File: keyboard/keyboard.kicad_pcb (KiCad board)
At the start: 2 copper layers, 166.5 x 124 mm, 82 parts, among them J1 Conn_01x04, J2 Conn_01x04, SW1 SW_Push, SW10 SW_Push, SW11 SW_Push, SW12 SW_Push, SW13 SW_Push, SW14 SW_Push, SW15 SW_Push, SW16 SW_Push, SW17 SW_Push, SW18 SW_Push, SW19 SW_Push, SW2 SW_Push, SW20 SW_Push, SW21 SW_Push, SW3 SW_Push, SW4 SW_Push, SW5 SW_Push, SW6 SW_Push, SW7 SW_Push, SW8 SW_Push, SW9 SW_Push, U1 AP2127K-3.3, U2 USBLC6-2SC6, U3 STM32F072CBTx

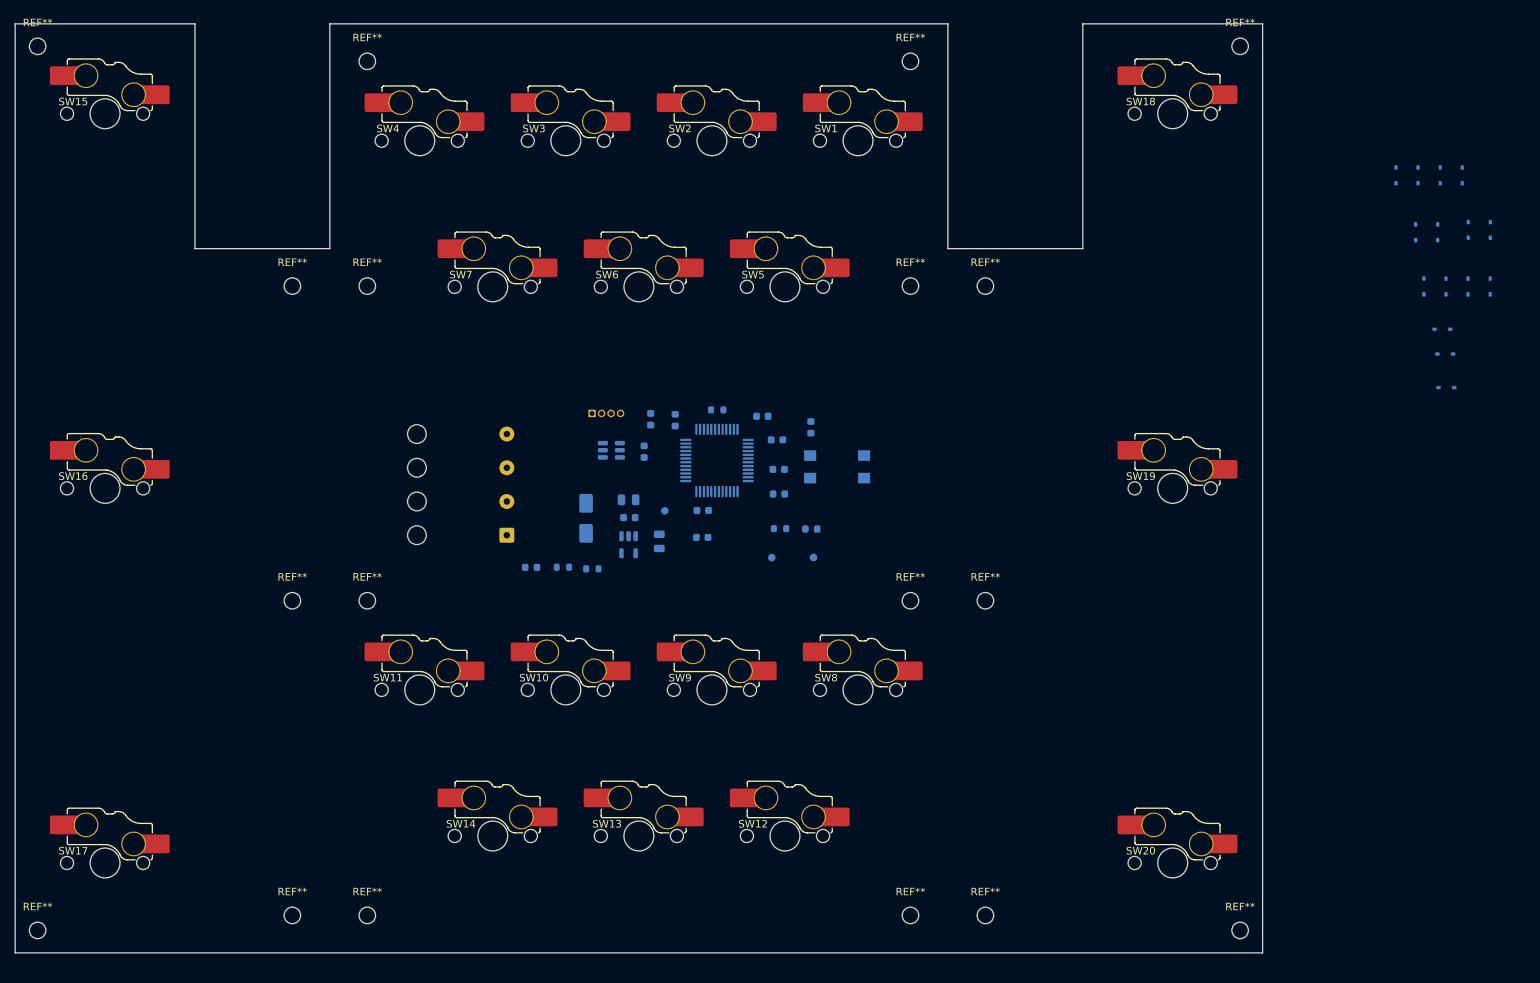
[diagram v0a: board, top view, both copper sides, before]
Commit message: Some switch traces.
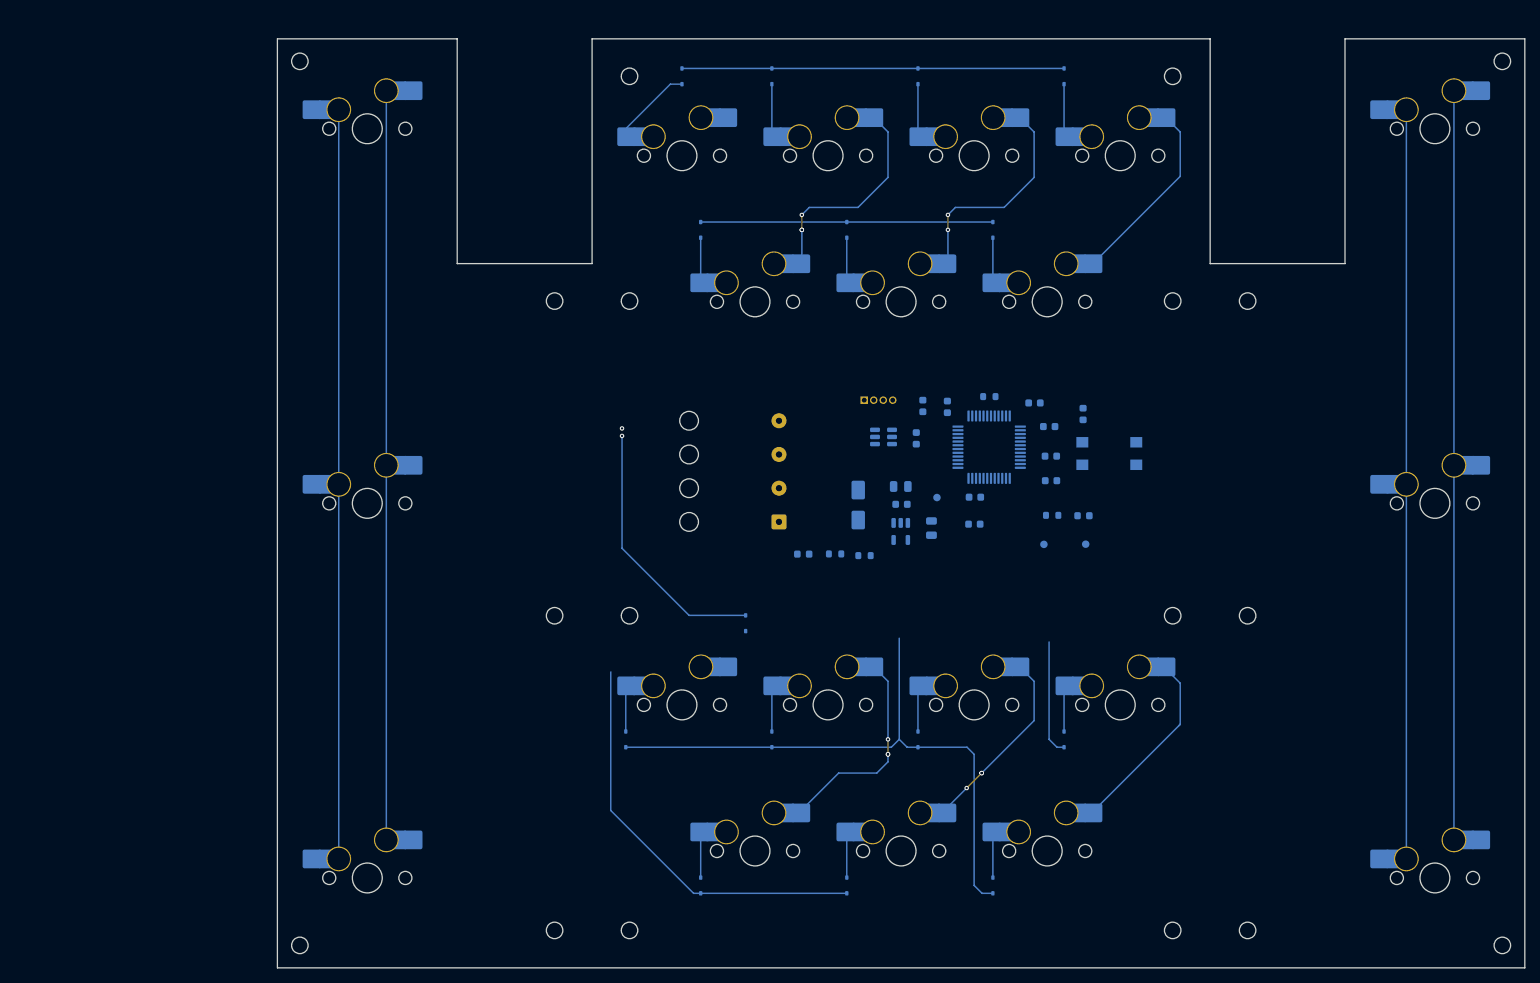
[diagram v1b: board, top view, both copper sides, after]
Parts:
- SW1, SW10, SW11, SW12, SW13, SW14, SW15, SW16, SW17, SW18, SW19, SW2, SW20, SW3, SW4, SW5, SW6, SW7, SW8, SW9: moved to B.Cu
- moved D14 127.6 mm to (111.5, 128.5), turned to 90 degrees
- moved D17 122.1 mm to (121.5, 148.0), turned to 90 degrees
- moved D16 108.8 mm to (141.0, 148.0), turned to 90 degrees
- moved D13 108.4 mm to (131.0, 128.5), turned to 90 degrees
- moved D7 105.0 mm to (119.0, 40.0)
- moved D15 103.9 mm to (160.5, 148.0), turned to 90 degrees
- moved D10 102.4 mm to (121.5, 60.5)
- moved D18 98.7 mm to (127.5, 113.0), turned to 90 degrees
- moved D12 90.6 mm to (150.5, 128.5), turned to 90 degrees
- moved D6 90.2 mm to (131.0, 40.0)
- moved D11 88.7 mm to (170.0, 128.5), turned to 90 degrees
- moved D9 78.9 mm to (141.0, 60.5)
- moved D5 68.0 mm to (150.5, 40.0)
- moved D8 56.4 mm to (160.5, 60.5)
- moved D4 46.2 mm to (170.0, 40.0)
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- renumbered REF** to ?
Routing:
- net Net-(D18-A): track 0.00 -> 235.2 mm, vias 0 -> 1
- net /COL3: track 0.00 -> 226.0 mm, vias 0 -> 1
- net /ROW2: track 0.00 -> 81.7 mm
- net /COL1: track 0.00 -> 56.8 mm, vias 0 -> 5
- net /ROW3: track 0.00 -> 54.6 mm
- net /ROW1: track 0.00 -> 54.4 mm
- net /ROW0: track 0.00 -> 51.0 mm
- net /COL0: track 0.00 -> 50.2 mm, vias 0 -> 3
- net /COL2: track 0.00 -> 29.0 mm, vias 0 -> 3
- net Net-(D7-A): track 0.00 -> 11.0 mm
- net Net-(D6-A): track 0.00 -> 7.07 mm
- net Net-(D5-A): track 0.00 -> 7.07 mm
- net Net-(D4-A): track 0.00 -> 7.07 mm
- net Net-(D14-A): track 0.00 -> 6.15 mm
- net Net-(D13-A): track 0.00 -> 6.15 mm
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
